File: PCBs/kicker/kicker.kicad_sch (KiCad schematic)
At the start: 33 parts, among them J2 Conn_01x04_Socket, J3 Conn_01x01_Socket, J4 Conn_01x01_Socket, Q1 CSD19534Q5A, U1 UCC27624DR, U2 XL6019E1

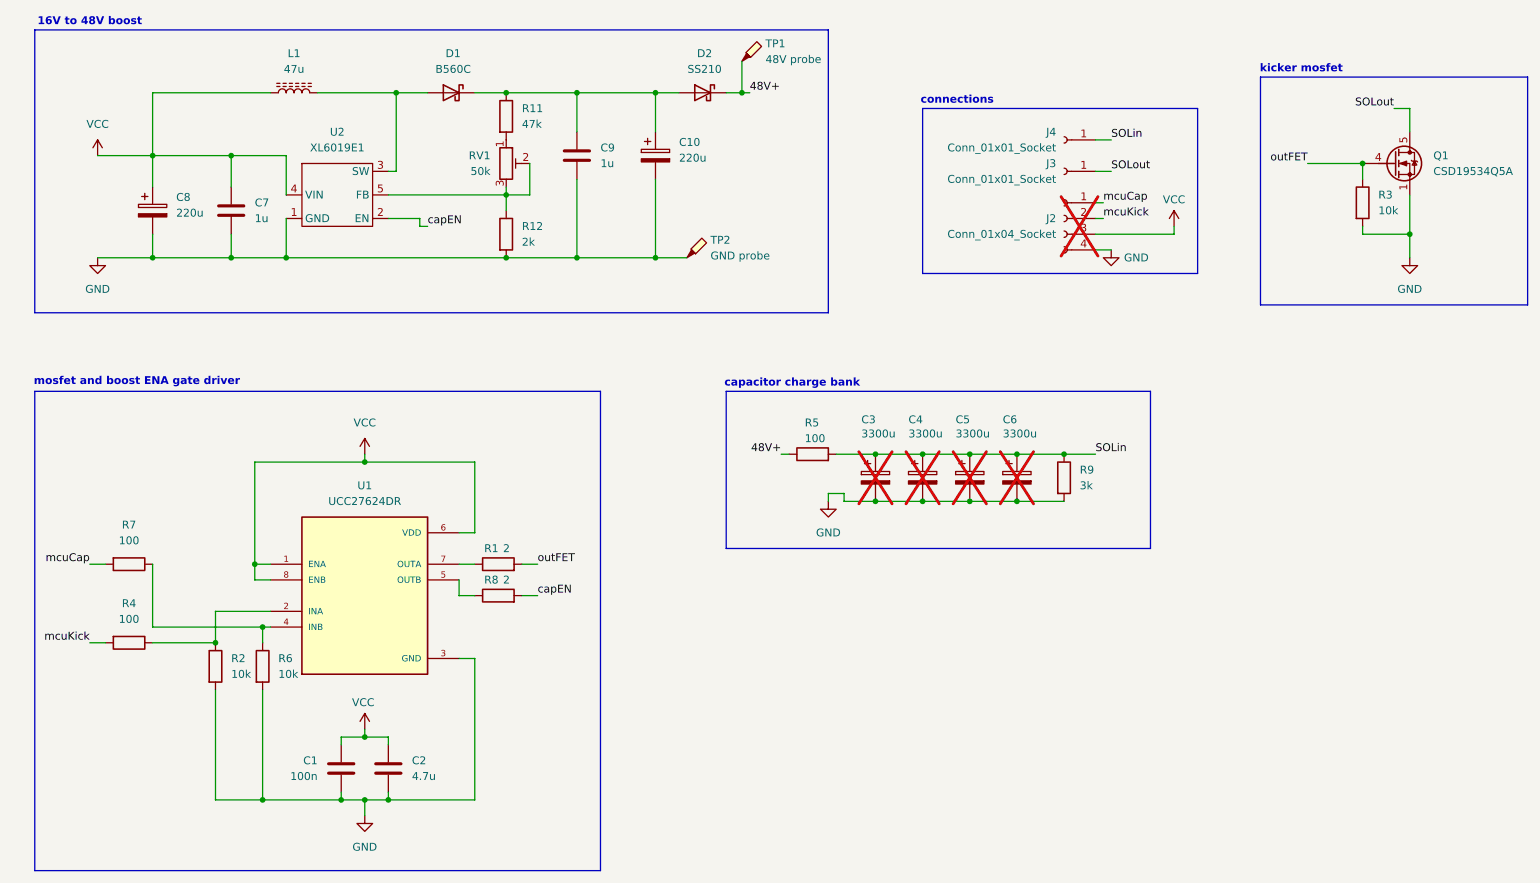
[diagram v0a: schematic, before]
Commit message: kicker v2 review
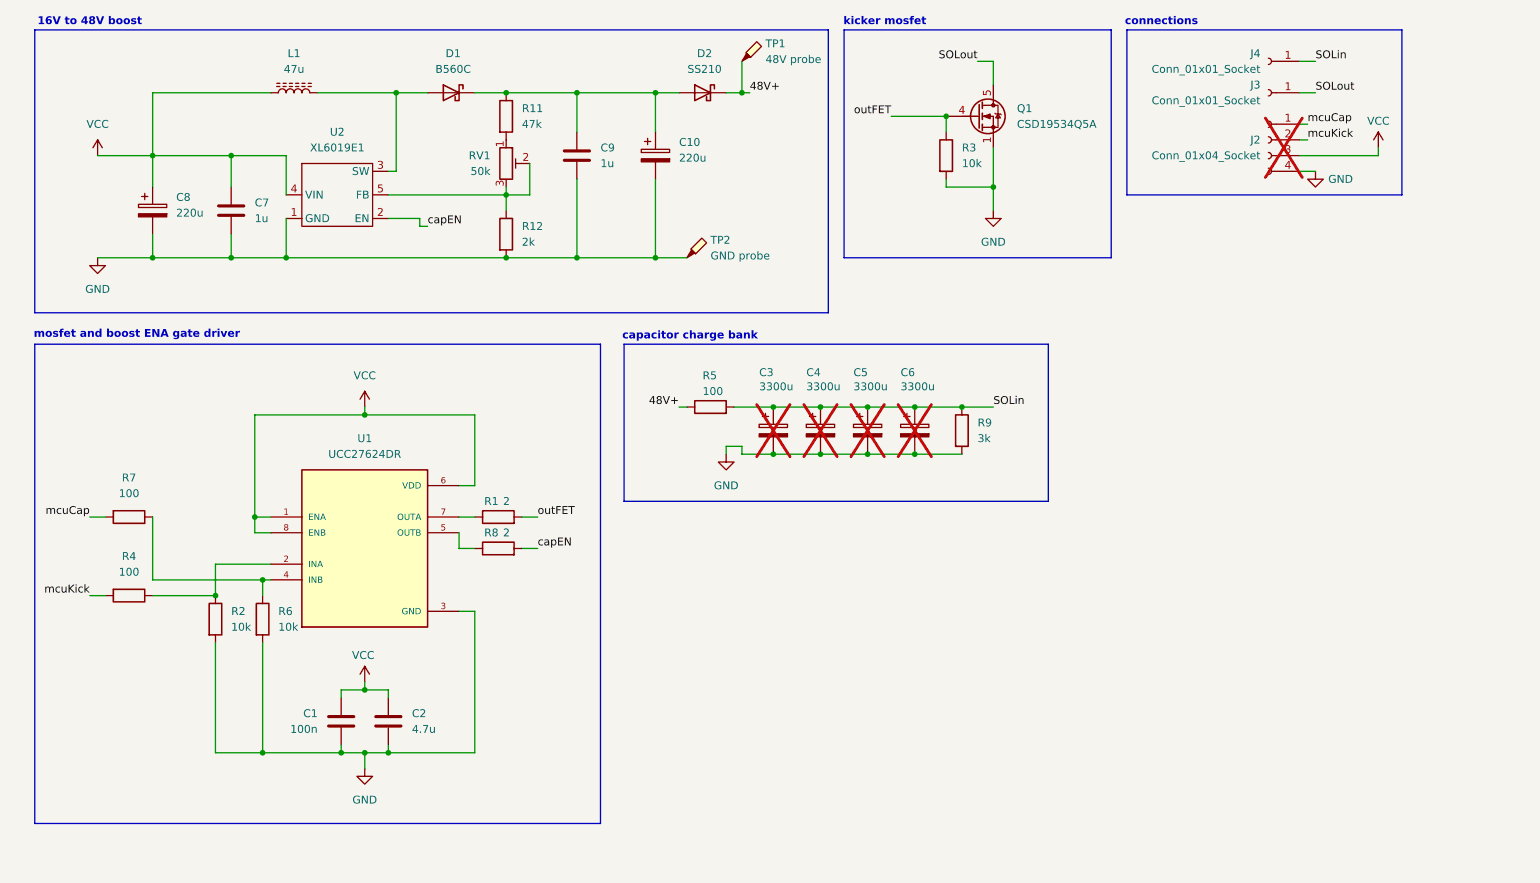
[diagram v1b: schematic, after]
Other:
- moved on the sheet: C1, C2, C3, C4, C5, C6, J2, J3, J4, Q1, R1, R2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
